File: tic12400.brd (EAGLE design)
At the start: 100 x 80 mm, 21 parts, among them U1 TIC12400DCPR, X1 22-23-2031

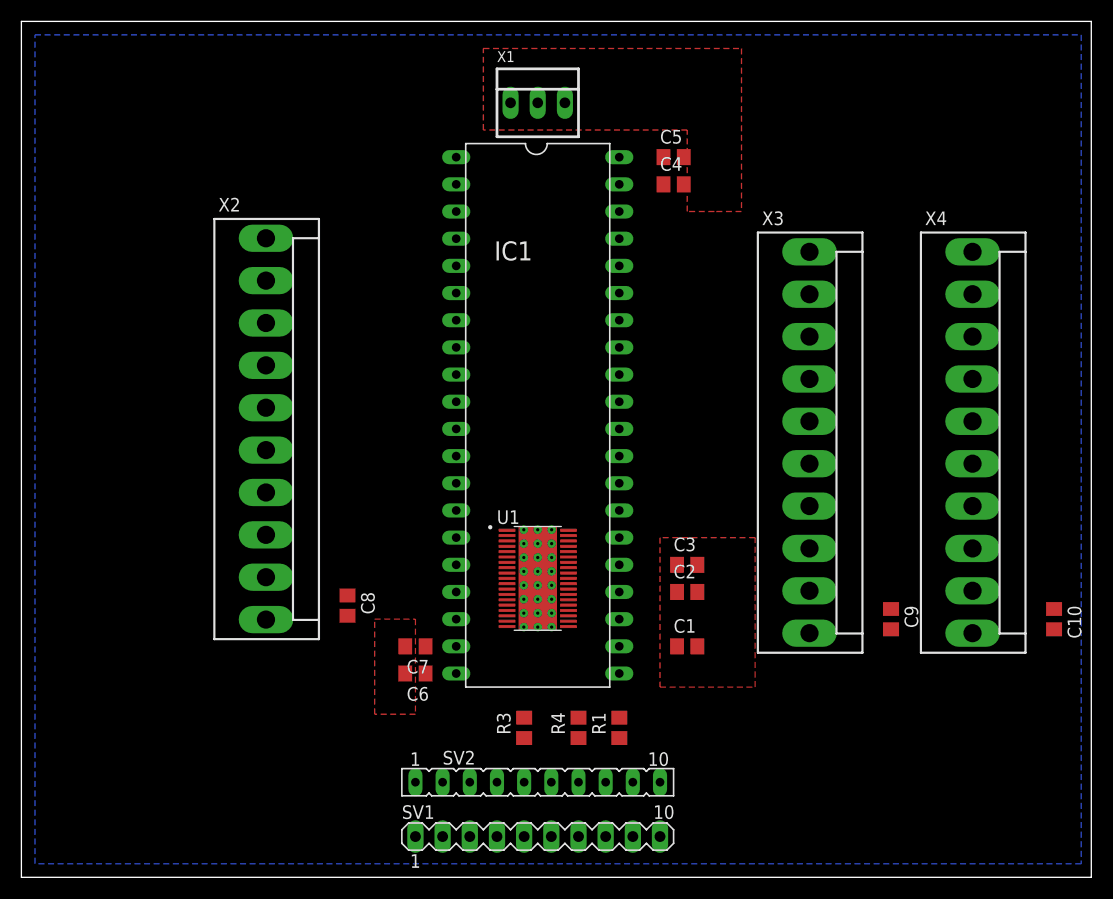
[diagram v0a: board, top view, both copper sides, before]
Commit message: up
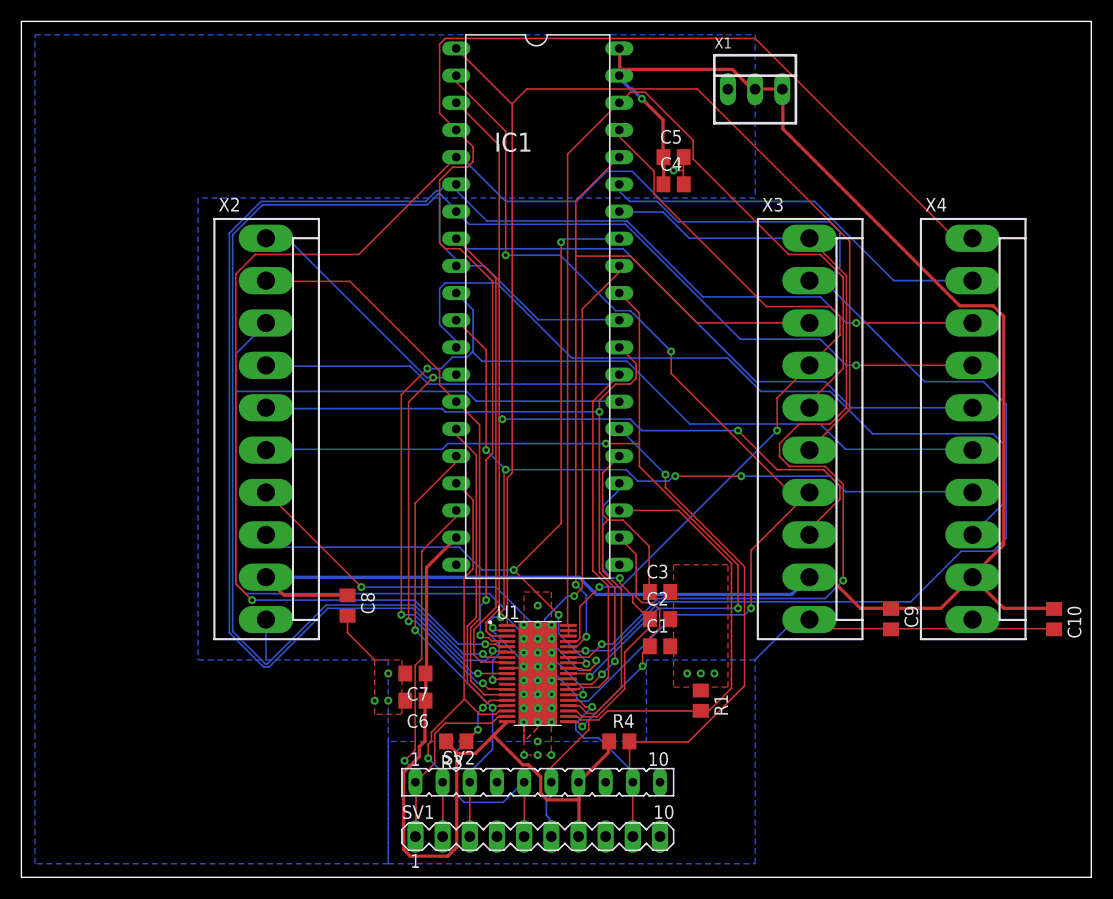
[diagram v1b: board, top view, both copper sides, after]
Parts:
- moved X1 20.4 mm to (68.6, 73.7)
- moved IC1 10.2 mm to (48.3, 53.3)
- moved U1 8.89 mm to (48.3, 19.1)
- moved R1 8.03 mm to (63.5, 16.5), turned to 270 degrees
- moved R3 6.48 mm to (40.6, 12.7), turned to 180 degrees
- moved R4 4.02 mm to (55.9, 12.7), turned to 0 degrees
- moved C2 3.59 mm to (59.7, 24.1)
- moved C3 3.59 mm to (59.7, 26.7)
- moved C1 2.54 mm to (59.7, 21.6)
- moved C6 2.54 mm to (36.8, 16.5)
- moved C7 2.54 mm to (36.8, 19.1)
- moved X3 1.27 mm to (73.7, 41.9)
- moved X4 1.27 mm to (88.9, 41.9)
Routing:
- net +24V: track 0.00 -> 175.4 mm, vias 0 -> 1
- net N$11: track 0.00 -> 146.6 mm, vias 0 -> 2
- net N$7: track 0.00 -> 145.7 mm, vias 0 -> 2
- net N$12: track 0.00 -> 137.2 mm, vias 0 -> 2
- net N$13: track 0.00 -> 122.5 mm, vias 0 -> 2
- net GND: track 0.00 -> 121.1 mm, vias 0 -> 12
- net N$16: track 0.00 -> 115.4 mm
- net N$24: track 0.00 -> 110.6 mm, vias 0 -> 1
- net N$15: track 0.00 -> 104.0 mm, vias 0 -> 4
- net N$17: track 0.00 -> 101.3 mm, vias 0 -> 1
- net N$5: track 0.00 -> 99.5 mm
- net N$3: track 0.00 -> 97.8 mm, vias 0 -> 3
- net N$27: track 0.00 -> 94.9 mm
- net N$14: track 0.00 -> 93.9 mm, vias 0 -> 2
- net N$23: track 0.00 -> 89.6 mm, vias 0 -> 2
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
